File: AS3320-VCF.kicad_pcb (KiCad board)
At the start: 2 copper layers, 67.2 x 91.3 mm, 41 parts, among them J1 SIGNAL_INPUT, J2 RESONANCE_CTRL_INPUT, J3 FREQ_CTRL_INPUT, J4 SIGNAL_OUTPUT, U1 AS3320

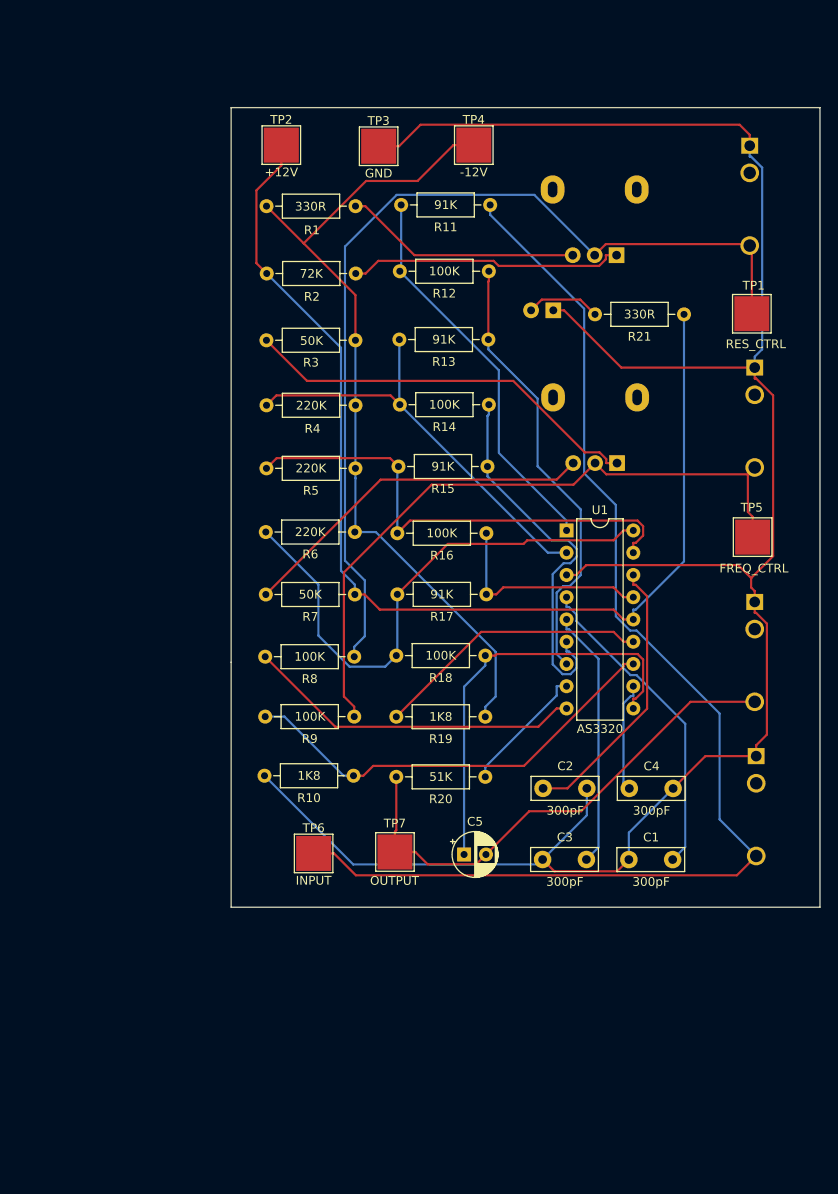
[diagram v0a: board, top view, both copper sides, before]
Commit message: Refactor
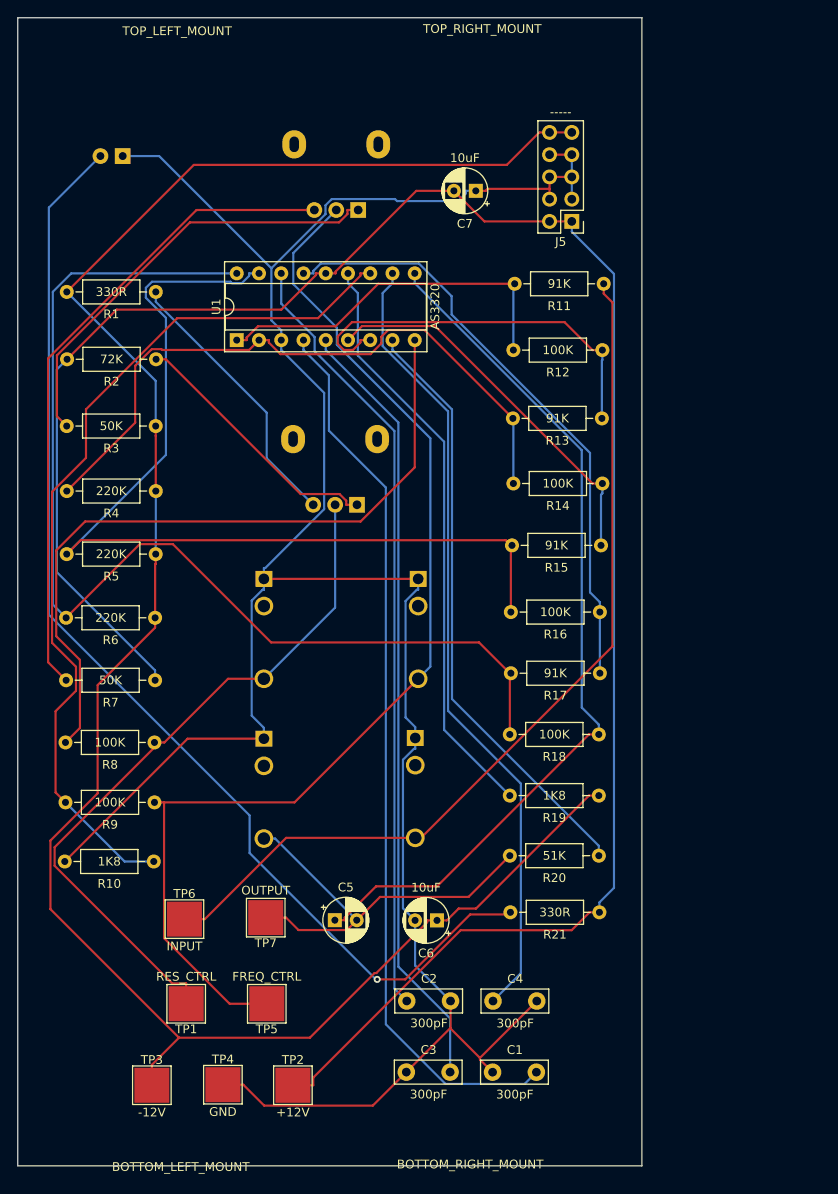
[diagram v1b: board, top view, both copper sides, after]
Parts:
- added BOTTOM_LEFT_MOUNT: MountingHole_3.2mm_M3_Oval, Seattle_Synths:MountingHole_3.2mm_M3_Oval, F.Cu at (109.1, 153.8)
- added BOTTOM_RIGHT_MOUNT: MountingHole_3.2mm_M3_Oval, Seattle_Synths:MountingHole_3.2mm_M3_Oval, F.Cu at (166.1, 154.0)
- added C6: 10uF, Seattle_Synths:CP_Radial_D5.0mm_P2.50mm, F.Cu at (149.6, 128.7)
- added C7: 10uF, Seattle_Synths:CP_Radial_D5.0mm_P2.50mm, F.Cu at (154.1, 45.4)
- added J5: -----, Seattle_Synths:PinHeader_2x05_P2.54mm_Vertical, F.Cu at (165.0, 48.9)
- added TOP_LEFT_MOUNT: MountingHole_3.2mm_M3_Oval, Seattle_Synths:MountingHole_3.2mm_M3_Oval, F.Cu at (109.2, 28.8)
- added TOP_RIGHT_MOUNT: MountingHole_3.2mm_M3_Oval, Seattle_Synths:MountingHole_3.2mm_M3_Oval, F.Cu at (166.0, 28.8)
- C1, C2, C3, C4: footprint SeattleSynths:C_Disc_D7.5mm_W2.5mm_P5.00mm -> Seattle_Synths:C_Disc_D7.5mm_W2.5mm_P5.00mm
- C5: footprint SeattleSynths:CP_Radial_D5.0mm_P2.50mm -> Seattle_Synths:CP_Radial_D5.0mm_P2.50mm
- D1: footprint SeattleSynths:LED_D5.0mm -> Seattle_Synths:LED_D5.0mm
- J1, J2, J3, J4: footprint SeattleSynths:Jack_3.5mm_QingPu_WQP-PJ398SM_Vertical_CircularHoles -> Seattle_Synths:Jack_3.5mm_QingPu_WQP-PJ398SM_Vertical_CircularHoles
- R1, R10, R11, R12, R13, R14, R15, R16, R17, R18, R19, R2, R20, R21, R3, R4, R5, R6, R7, R8, R9: footprint SeattleSynths:R_Axial_DIN0207_L6.3mm_D2.5mm_P10.16mm_Horizontal -> Seattle_Synths:R_Axial_DIN0207_L6.3mm_D2.5mm_P10.16mm_Horizontal
- RV1, RV2: footprint SeattleSynths:Potentiometer_Alpha_RD901F-40-00D_Single_Vertical -> Seattle_Synths:Potentiometer_Alpha_RD901F-40-00D_Single_Vertical
- TP1, TP2, TP5, TP6, TP7: footprint SeattleSynths:TestPoint_Pad_4.0x4.0mm -> Seattle_Synths:TestPoint_Pad_4.0x4.0mm
- TP3: value GND -> -12V; footprint SeattleSynths:TestPoint_Pad_4.0x4.0mm -> Seattle_Synths:TestPoint_Pad_4.0x4.0mm
- TP4: value -12V -> GND; footprint SeattleSynths:TestPoint_Pad_4.0x4.0mm -> Seattle_Synths:TestPoint_Pad_4.0x4.0mm
- U1: footprint SeattleSynths:DIP-18_W7.62mm -> Seattle_Synths:DIP-18_W7.62mm_Socket
- moved TP4 111.0 mm to (125.2, 147.4)
- moved TP3 110.3 mm to (117.1, 147.5)
- moved TP2 107.3 mm to (133.2, 147.5)
- moved TP1 101.9 mm to (121.0, 138.2)
- moved TP5 76.9 mm to (130.2, 138.2)
- moved J2 74.3 mm to (129.9, 89.7)
- moved R21 68.9 mm to (158.0, 127.8)
- moved J4 58.2 mm to (129.9, 108.0)
- moved D1 52.2 mm to (113.8, 41.4)
- moved J3 45.4 mm to (147.5, 89.7)
- moved U1 43.5 mm to (126.8, 62.5), turned to 90 degrees
- moved RV2 41.3 mm to (140.6, 47.6)
- moved RV1 41.1 mm to (140.5, 81.2)
- moved J1 39.0 mm to (147.2, 107.9)
- moved C1 28.8 mm to (156.0, 146.0)
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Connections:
- TP3 pad 1: GND -> -12V
- TP4 pad 1: -12V -> GND
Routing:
- net -12V: track 95.1 -> 231.8 mm
- net Net-(D1-Pad2): track 8.51 -> 130.4 mm, vias 0 -> 1
- net +12V: track 127.5 -> 234.3 mm
- net Net-(C4-Pad1): track 12.6 -> 91.4 mm
- net Net-(C1-Pad2): track 36.7 -> 102.6 mm
- net Net-(R17-Pad1): track 62.2 -> 127.1 mm
- net Net-(C3-Pad2): track 29.7 -> 89.4 mm
- net Net-(C2-Pad1): track 31.7 -> 89.0 mm
- net /VRES: track 14.8 -> 68.6 mm
- net Net-(R15-Pad1): track 56.2 -> 109.3 mm
- net /OUT4: track 48.3 -> 100.4 mm
- net /FREQ_CTRL_INPUT: track 77.3 -> 128.9 mm
- net Net-(R10-Pad2): track 50.3 -> 101.0 mm
- net /OUT3: track 24.6 -> 69.1 mm
- net Net-(R8-Pad1): track 38.6 -> 83.1 mm
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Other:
- board size 67.2 x 91.3 mm -> 71.2 x 131.1 mm
- board text added: "Seattle Synths SS-VCF-1 Rev. 1 [2020-11-08]"
- board text added: "This machine kills fascists."
